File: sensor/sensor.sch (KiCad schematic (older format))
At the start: 37 parts, among them J1 Conn_01x08_Female, U1 DHT22, U2 SSCDRNN015PASA5, U3 TCA9555DBR

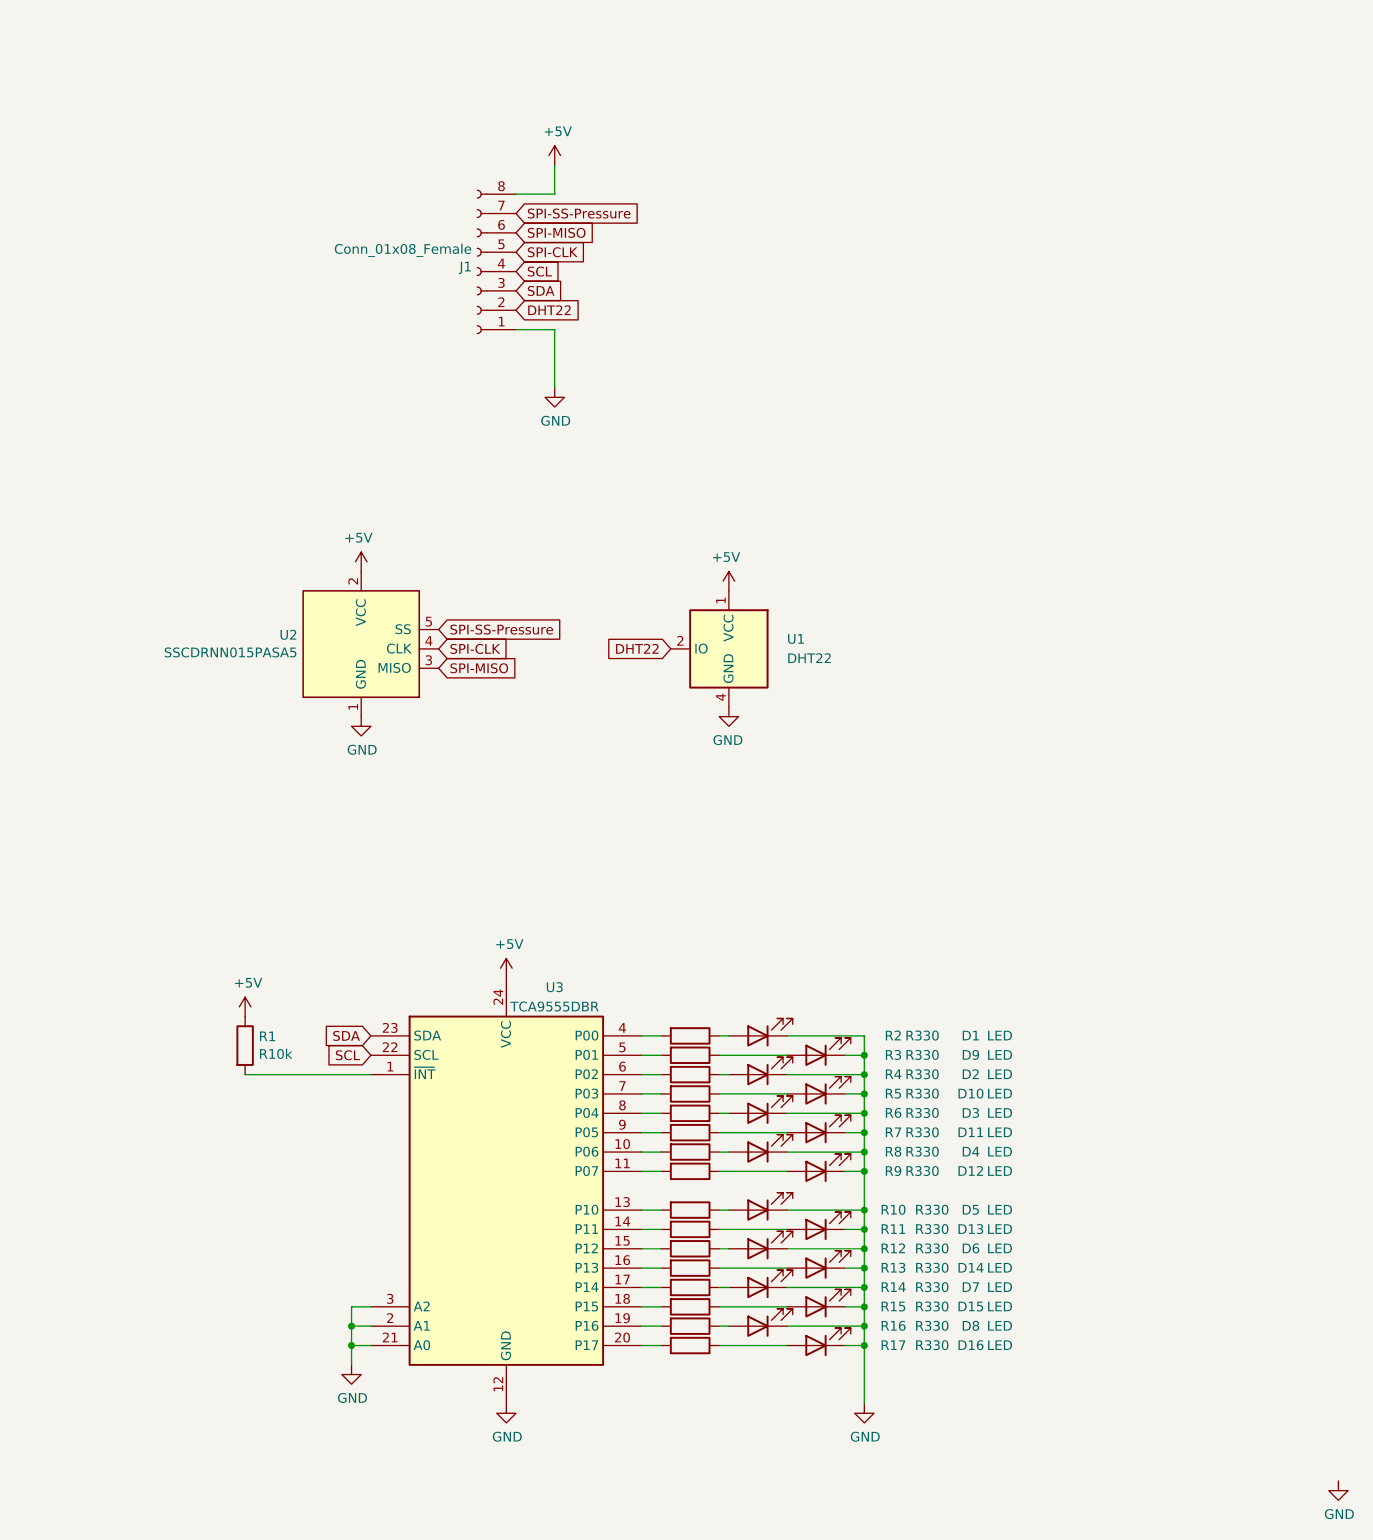
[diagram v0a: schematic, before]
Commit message: change everything
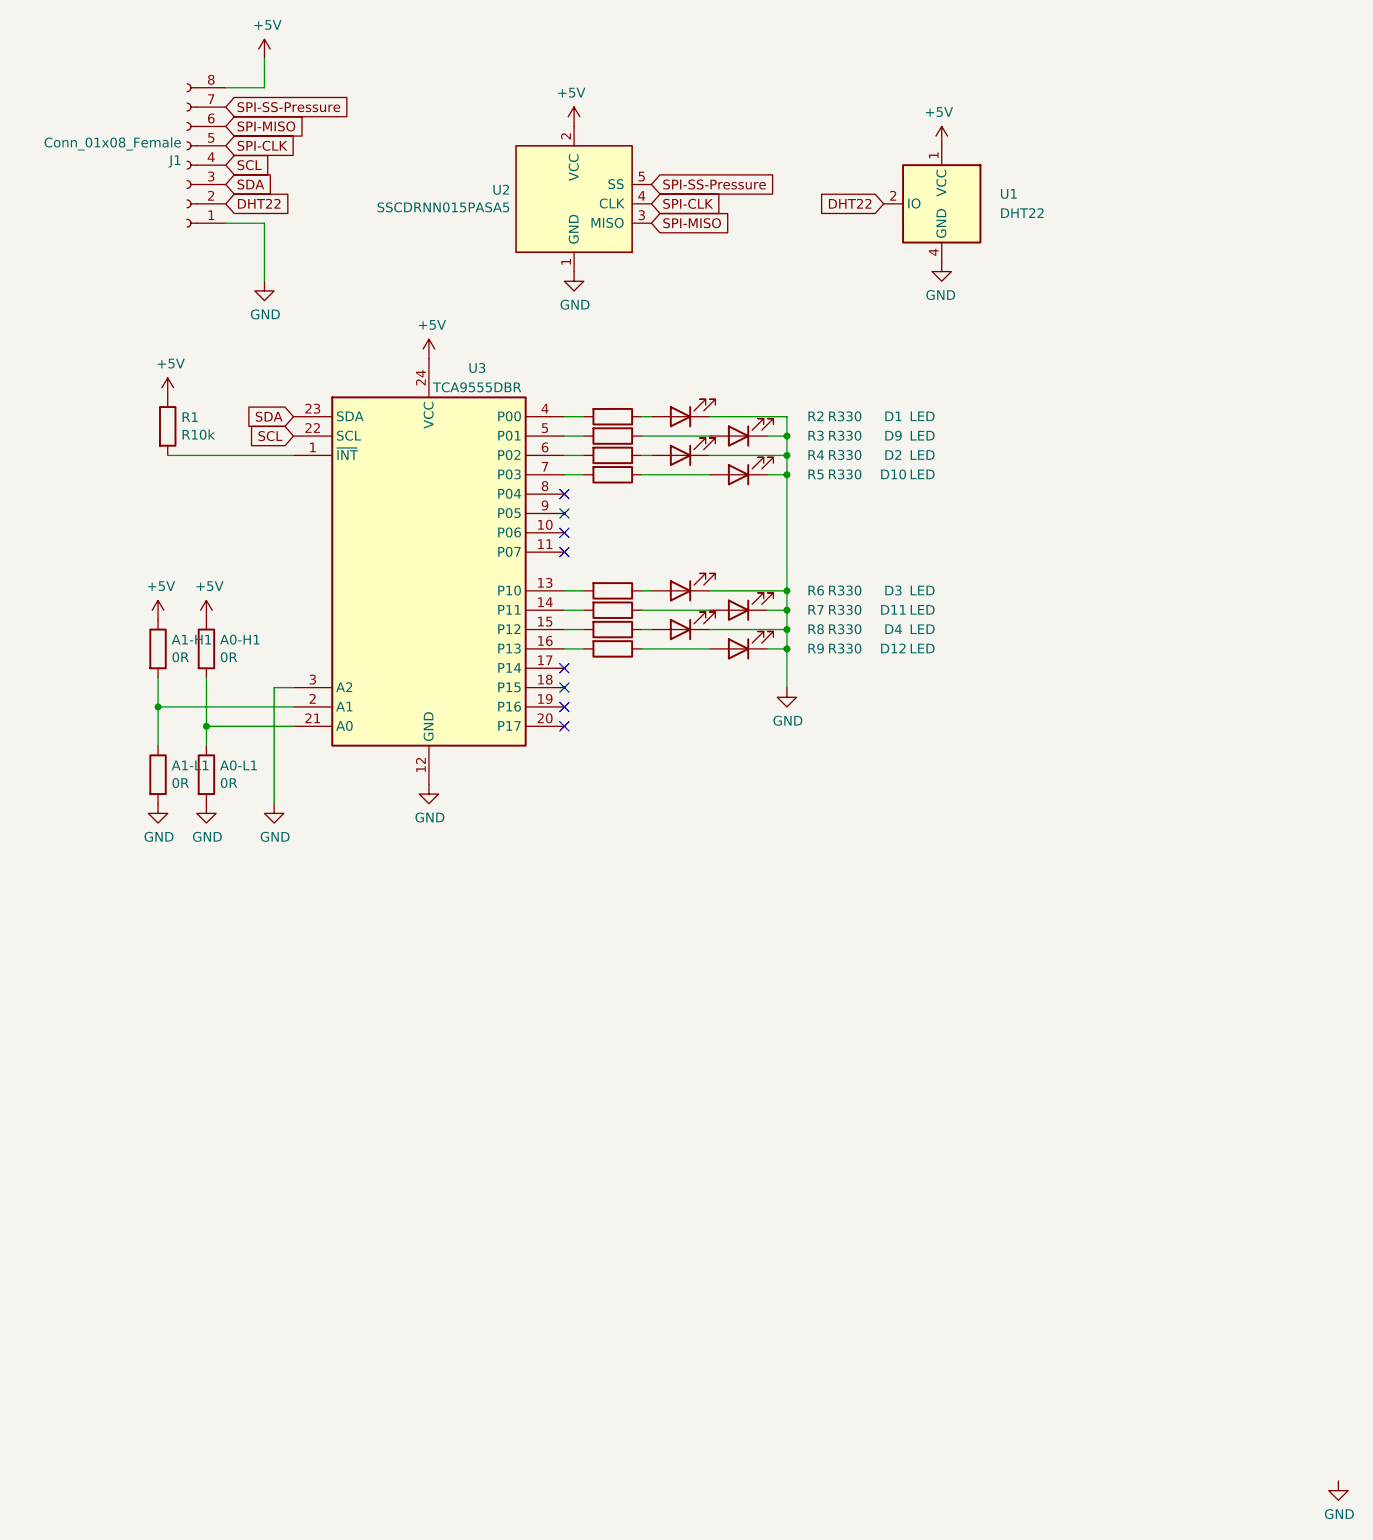
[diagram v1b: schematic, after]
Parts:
- removed D13, D14, D15, D16, D5, D6, D7, D8: LED, LED_SMD:LED_0805_2012Metric_Pad1.15x1.40mm_HandSolder, symbol Device:LED
- removed R10, R11, R12, R13, R14, R15, R16, R17: R330, Resistor_SMD:R_0603_1608Metric, symbol Device:R
- added A0-H1, A0-L1, A1-H1, A1-L1: 0R, Resistor_SMD:R_0603_1608Metric_Pad0.98x0.95mm_HandSolder, symbol Device:R
- D1, D10, D11, D12, D2, D3, D4, D9: footprint LED_SMD:LED_0805_2012Metric_Pad1.15x1.40mm_HandSolder -> LED_THT:LED_D5.0mm
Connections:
- net +5V: now also A0-H1.1, A1-H1.1
- net GND: now also A0-L1.2, A1-L1.2; no longer U3.2 (A1), U3.21 (A0)
- net at R6.2: now also U3.13 (P10); no longer U3.8 (P04)
- net at R7.2: now also U3.14 (P11); no longer U3.9 (P05)
- net at R8.2: now also U3.15 (P12); no longer U3.10 (P06)
- net at R9.2: now also U3.16 (P13); no longer U3.11 (P07)
- new net: A1-H1.2, A1-L1.1, U3.2 (A1)
- new net: A0-H1.2, A0-L1.1, U3.21 (A0)
- no-connect marks 0 -> 8
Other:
- moved on the sheet: D1, D10, D11, D12, D2, D3, D4, D9, J1, R1, R2, R3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
